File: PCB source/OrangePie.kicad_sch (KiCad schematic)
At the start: 0 parts

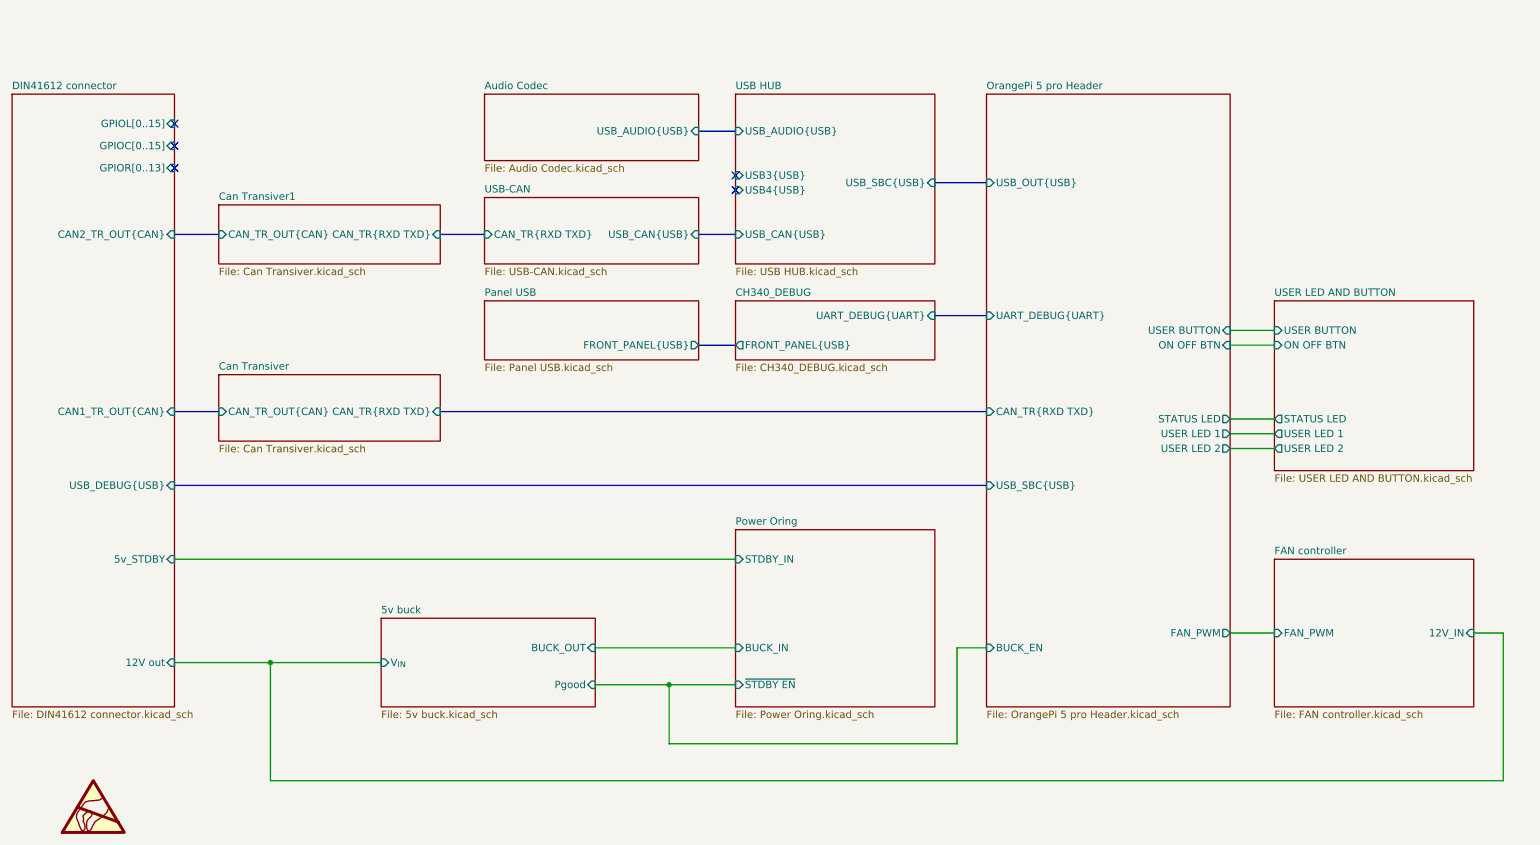
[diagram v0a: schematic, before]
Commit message: Fix schematic
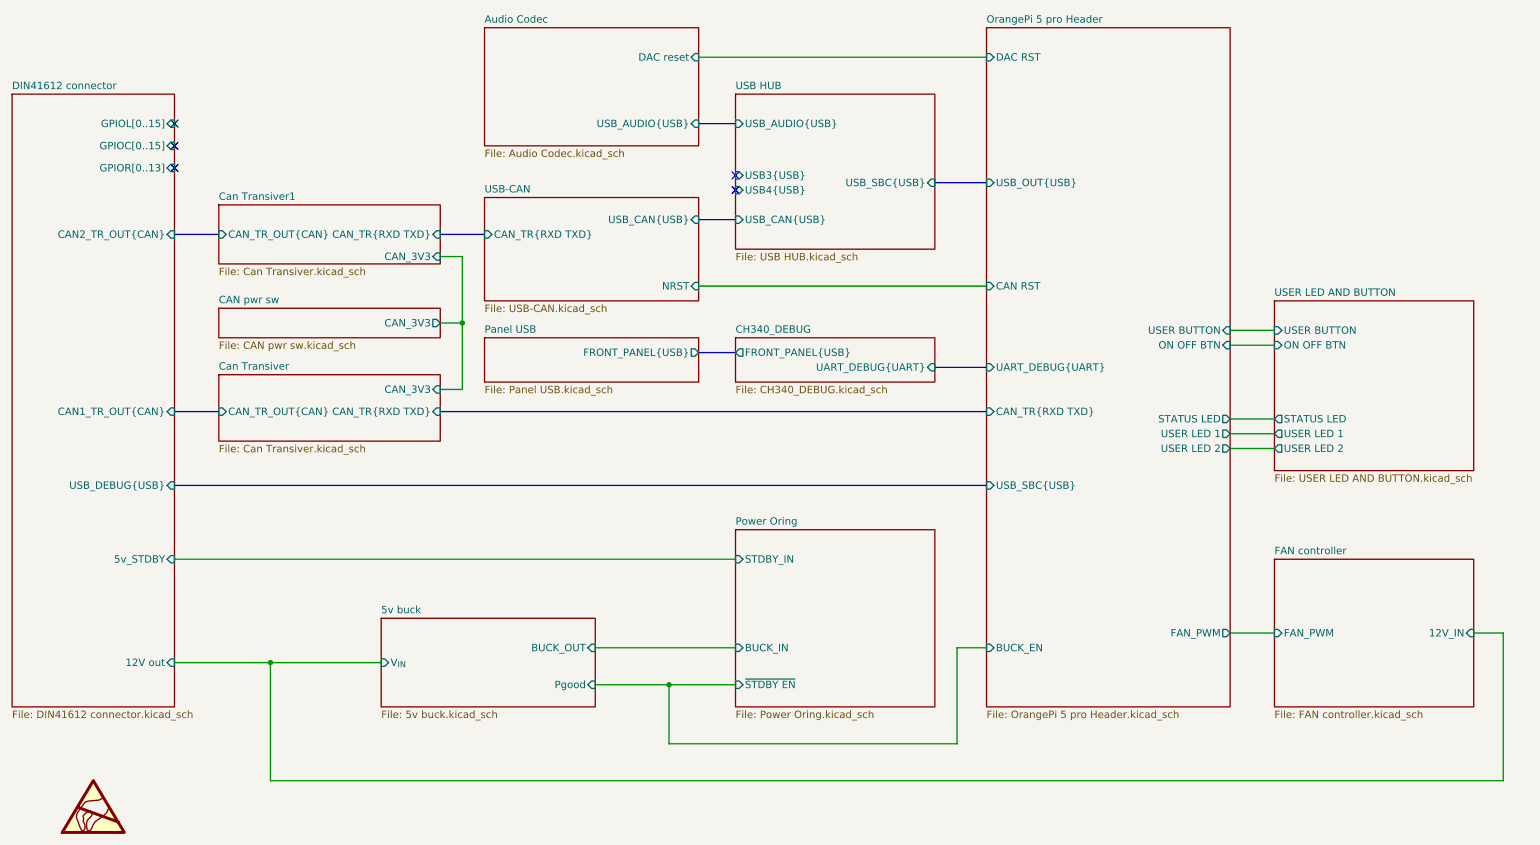
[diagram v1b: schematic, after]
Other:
- added sheet CAN pwr sw (CAN pwr sw.kicad_sch)
- sheet Audio Codec ports: added DAC reset; removed none
- sheet Can Transiver ports: added CAN_3V3; removed none
- sheet Can Transiver1 ports: added CAN_3V3; removed none
- sheet OrangePi 5 pro Header ports: added CAN RST, DAC RST; removed none
- sheet USB-CAN ports: added NRST; removed none
